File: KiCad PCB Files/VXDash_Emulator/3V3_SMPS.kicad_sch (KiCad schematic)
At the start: 13 parts, among them IC2 AP62200

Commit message: Emulator board : BOM and fab prep
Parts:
- C10: MFT (none) -> Samsung Electro-Mechanics; MFT_PN (none) -> CL31B106KAHNNNE
- C11, C12, C14: MFT (none) -> Samsung Electro-Mechanics; MFT_PN (none) -> CL10B104KB8NNWC
- C13: MFT (none) -> Kyocera AVX; MFT_PN (none) -> 06035C220JAT2A
- C15, C16: MFT (none) -> Samsung Electro-Mechanics; MFT_PN (none) -> CL31B226KPHNNNE
- R91: MFT (none) -> StackPole Electronics; MFT_PN (none) -> RMCF0603FT820K
- R92: MFT (none) -> StackPole Electronics; MFT_PN (none) -> RMCF0603FT120K
- R93: MFT (none) -> StackPole Electronics; MFT_PN (none) -> RMCF0603FT75K0
- R94: MFT (none) -> Yageo; MFT_PN (none) -> RC0603FR-1324KL
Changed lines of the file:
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@@
 			)
 		)
-		(property "Description" ""
+		(property "Description" "CAP CER 22PF 50V X7R 0603"
 			(at 168.91 66.04 0)
 			(effects
@@
 			)
 		)
-		(property "MFT" ""
+		(property "MFT" "Kyocera AVX"
 			(at 168.91 66.04 0)
 			(effects
@@
 			)
 		)
-		(property "MFT_PN" ""
+		(property "MFT_PN" "06035C220JAT2A"
 			(at 168.91 66.04 0)
 			(effects
@@
 			)
 		)
-		(property "Description" ""
+		(property "Description" "RES 24K OHM 1% 1/10W 0603"
 			(at 160.02 77.47 0)
 			(effects
@@
 			)
 		)
-		(property "MFT" ""
+		(property "MFT" "Yageo"
 			(at 160.02 77.47 0)
 			(effects
@@
 			)
 		)
-		(property "MFT_PN" ""
+		(property "MFT_PN" "RC0603FR-1324KL"
 			(at 160.02 77.47 0)
 			(effects
@@
 			)
 		)
-		(property "Description" ""
+		(property "Description" "CAP CER 10UF 25V X7R 1206"
 			(at 99.06 62.23 0)
 			(effects
@@
 			)
 		)
-		(property "MFT" ""
+		(property "MFT" "Samsung Electro-Mechanics"
 			(at 99.06 62.23 0)
 			(effects
@@
 			)
 		)
-		(property "MFT_PN" ""
+		(property "MFT_PN" "CL31B106KAHNNNE"
 			(at 99.06 62.23 0)
 			(effects
@@
 			)
 		)
-		(property "Description" ""
+		(property "Description" "RES 75K OHM 1% 1/10W 0603"
 			(at 160.02 66.04 0)
 			(effects
@@
 			)
 		)
-		(property "MFT" ""
+		(property "MFT" "StackPole Electronics"
 			(at 160.02 66.04 0)
 			(effects
@@
 			)
 		)
-		(property "MFT_PN" ""
+		(property "MFT_PN" "RMCF0603FT75K0"
 			(at 160.02 66.04 0)
 			(effects
@@
 			)
 		)
-		(property "Description" ""
+		(property "Description" "RES 820K OHM 1% 1/10W 0603"
 			(at 88.9 63.5 0)
 			(effects
@@
 			)
 		)
-		(property "MFT" ""
+		(property "MFT" "StackPole Electronics"
 			(at 88.9 63.5 0)
 			(effects
@@
 			)
 		)
-		(property "MFT_PN" ""
+		(property "MFT_PN" "RMCF0603FT820K"
 			(at 88.9 63.5 0)
 			(effects
@@
 			)
 		)
-		(property "Description" ""
+		(property "Description" "CAP CER 22UF 10V X7R 1206"
 			(at 200.66 66.04 0)
 			(effects
@@
 			)
 		)
-		(property "MFT" ""
+		(property "MFT" "Samsung Electro-Mechanics"
 			(at 200.66 66.04 0)
 			(effects
@@
 			)
 		)
-		(property "MFT_PN" ""
+		(property "MFT_PN" "CL31B226KPHNNNE"
 			(at 200.66 66.04 0)
 			(effects
@@
 			)
 		)
-		(property "Description" ""
+		(property "Description" "CAP CER 22UF 10V X7R 1206"
 			(at 193.04 66.04 0)
 			(effects
@@
 			)
 		)
-		(property "MFT" ""
+		(property "MFT" "Samsung Electro-Mechanics"
 			(at 193.04 66.04 0)
 			(effects
@@
 			)
 		)
-		(property "MFT_PN" ""
+		(property "MFT_PN" "CL31B226KPHNNNE"
 			(at 193.04 66.04 0)
 			(effects
@@
 			)
 		)
-		(property "Description" ""
+		(property "Description" "FIXED IND 3.3UH 3A 30 MOHM SMD"
 			(at 153.67 63.5 0)
 			(effects
@@
 			)
 		)
-		(property "Description" ""
+		(property "Description" "RES 120K OHM 1% 1/10W 0603"
 			(at 88.9 76.2 0)
 			(effects
@@
 			)
 		)
-		(property "MFT" ""
+		(property "MFT" "StackPole Electronics"
 			(at 88.9 76.2 0)
 			(effects
@@
 			)
 		)
-		(property "MFT_PN" ""
+		(property "MFT_PN" "RMCF0603FT120K"
 			(at 88.9 76.2 0)
 			(effects
@@
 			)
 		)
-		(property "Description" ""
+		(property "Description" "CAP CER 0.1UF 50V X7R 0603"
 			(at 106.68 62.23 0)
 			(effects
@@
 			)
 		)
-		(property "MFT" ""
+		(property "MFT" "Samsung Electro-Mechanics"
 			(at 106.68 62.23 0)
 			(effects
@@
 			)
 		)
-		(property "MFT_PN" ""
+		(property "MFT_PN" "CL10B104KB8NNWC"
 			(at 106.68 62.23 0)
 			(effects
@@
 			)
 		)
-		(property "Description" ""
+		(property "Description" "CAP CER 0.1UF 50V X7R 0603"
 			(at 140.97 55.88 0)
 			(effects
@@
 			)
 		)
-		(property "MFT" ""
+		(property "MFT" "Samsung Electro-Mechanics"
 			(at 140.97 55.88 0)
 			(effects
@@
 			)
 		)
-		(property "MFT_PN" ""
+		(property "MFT_PN" "CL10B104KB8NNWC"
 			(at 140.97 55.88 0)
 			(effects
@@
 			)
 		)
-		(property "Description" ""
+		(property "Description" "CAP CER 0.1UF 50V X7R 0603"
 			(at 185.42 66.04 0)
 			(effects
@@
 			)
 		)
-		(property "MFT" ""
+		(property "MFT" "Samsung Electro-Mechanics"
 			(at 185.42 66.04 0)
 			(effects
@@
 			)
 		)
-		(property "MFT_PN" ""
+		(property "MFT_PN" "CL10B104KB8NNWC"
 			(at 185.42 66.04 0)
 			(effects

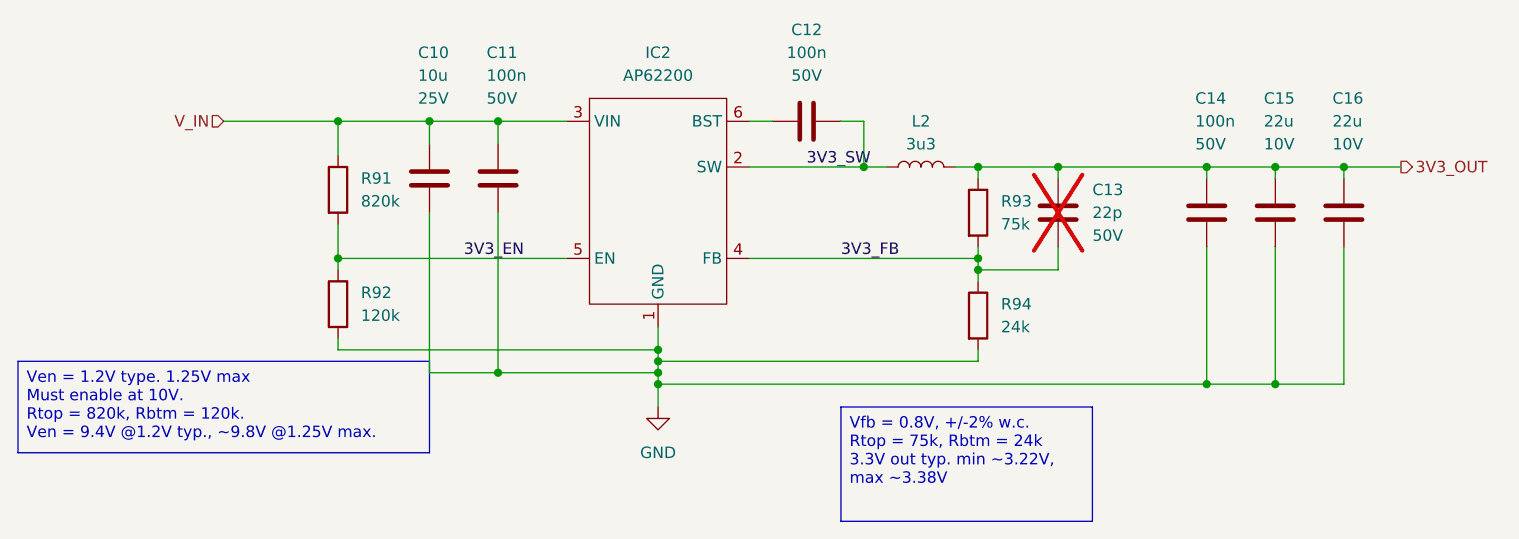
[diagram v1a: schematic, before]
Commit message: Emulator : LCSC part numbers and production files
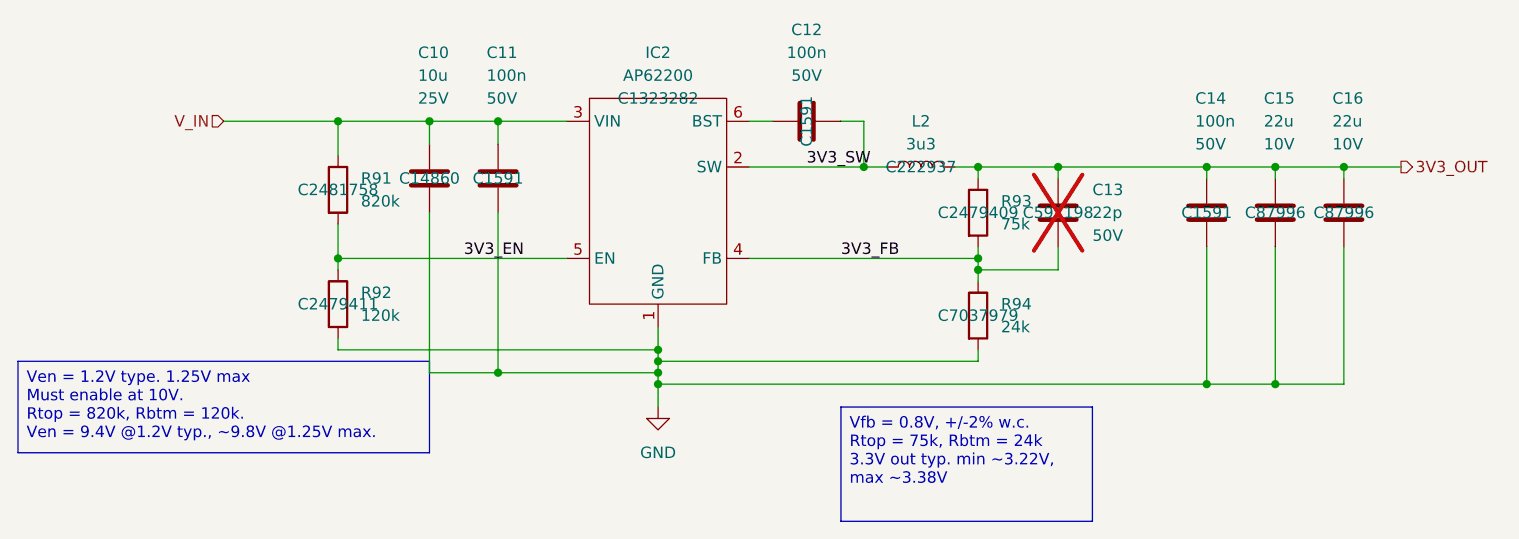
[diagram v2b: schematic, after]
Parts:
- C10: LCSC (none) -> C14860
- C11, C12, C14: LCSC (none) -> C1591; MFT_PN CL10B104KB8NNWC -> CL10B104KB8NNNC
- C13: LCSC (none) -> C597198
- C15, C16: LCSC (none) -> C87996
- IC2: LCSC (none) -> C1323282
- L2: LCSC (none) -> C222937
- R91: LCSC (none) -> C2481758
- R92: LCSC (none) -> C2479411
- R93: LCSC (none) -> C2479409
- R94: LCSC (none) -> C7037979
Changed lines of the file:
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@@
+			)
+		)
+		(property "LCSC" "C1323282"
+			(at 124.46 53.34 0)
+			(effects
+				(font
+					(size 1.27 1.27)
+				)
 			)
 		)
@@
 			)
 		)
+		(property "LCSC" "C597198"
+			(at 168.91 66.04 0)
+			(effects
+				(font
+					(size 1.27 1.27)
+				)
+			)
+		)
 		(pin "1"
 		)
@@
 			)
 		)
+		(property "LCSC" "C7037979"
+			(at 160.02 77.47 0)
+			(effects
+				(font
+					(size 1.27 1.27)
+				)
+			)
+		)
 		(pin "1"
 		)
@@
 			)
 		)
+		(property "LCSC" "C14860"
+			(at 99.06 62.23 0)
+			(effects
+				(font
+					(size 1.27 1.27)
+				)
+			)
+		)
 		(pin "1"
 		)
@@
 			)
 		)
+		(property "LCSC" "C2479409"
+			(at 160.02 66.04 0)
+			(effects
+				(font
+					(size 1.27 1.27)
+				)
+			)
+		)
 		(pin "1"
 		)
@@
 			)
 		)
+		(property "LCSC" "C2481758"
+			(at 88.9 63.5 0)
+			(effects
+				(font
+					(size 1.27 1.27)
+				)
+			)
+		)
 		(pin "1"
 		)
@@
 			)
 		)
+		(property "LCSC" "C87996"
+			(at 200.66 66.04 0)
+			(effects
+				(font
+					(size 1.27 1.27)
+				)
+			)
+		)
 		(pin "2"
 		)
@@
 				)
 				(hide yes)
+			)
+		)
+		(property "LCSC" "C87996"
+			(at 193.04 66.04 0)
+			(effects
+				(font
+					(size 1.27 1.27)
+				)
 			)
 		)
@@
 			)
 		)
+		(property "LCSC" "C222937"
+			(at 153.67 60.96 0)
+			(effects
+				(font
+					(size 1.27 1.27)
+				)
+			)
+		)
 		(pin "2"
 		)
@@
 			)
 		)
+		(property "LCSC" "C2479411"
+			(at 88.9 76.2 0)
+			(effects
+				(font
+					(size 1.27 1.27)
+				)
+			)
+		)
 		(pin "1"
 		)
@@
 			)
 		)
-		(property "MFT_PN" "CL10B104KB8NNWC"
+		(property "MFT_PN" "CL10B104KB8NNNC"
 			(at 106.68 62.23 0)
 			(effects
@@
 				)
 				(hide yes)
+			)
+		)
+		(property "LCSC" "C1591"
+			(at 106.68 62.23 0)
+			(effects
+				(font
+					(size 1.27 1.27)
+				)
 			)
 		)
@@
 			)
 		)
-		(property "MFT_PN" "CL10B104KB8NNWC"
+		(property "MFT_PN" "CL10B104KB8NNNC"
 			(at 140.97 55.88 0)
 			(effects
@@
 				)
 				(hide yes)
+			)
+		)
+		(property "LCSC" "C1591"
+			(at 140.97 55.88 0)
+			(effects
+				(font
+					(size 1.27 1.27)
+				)
 			)
 		)
@@
 			)
 		)
-		(property "MFT_PN" "CL10B104KB8NNWC"
+		(property "MFT_PN" "CL10B104KB8NNNC"
 			(at 185.42 66.04 0)
 			(effects
@@
 			)
 		)
+		(property "LCSC" "C1591"
+			(at 185.42 66.04 0)
+			(effects
+				(font
+					(size 1.27 1.27)
+				)
+			)
+		)

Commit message: Emulator : Updating BOM with LCSC alts
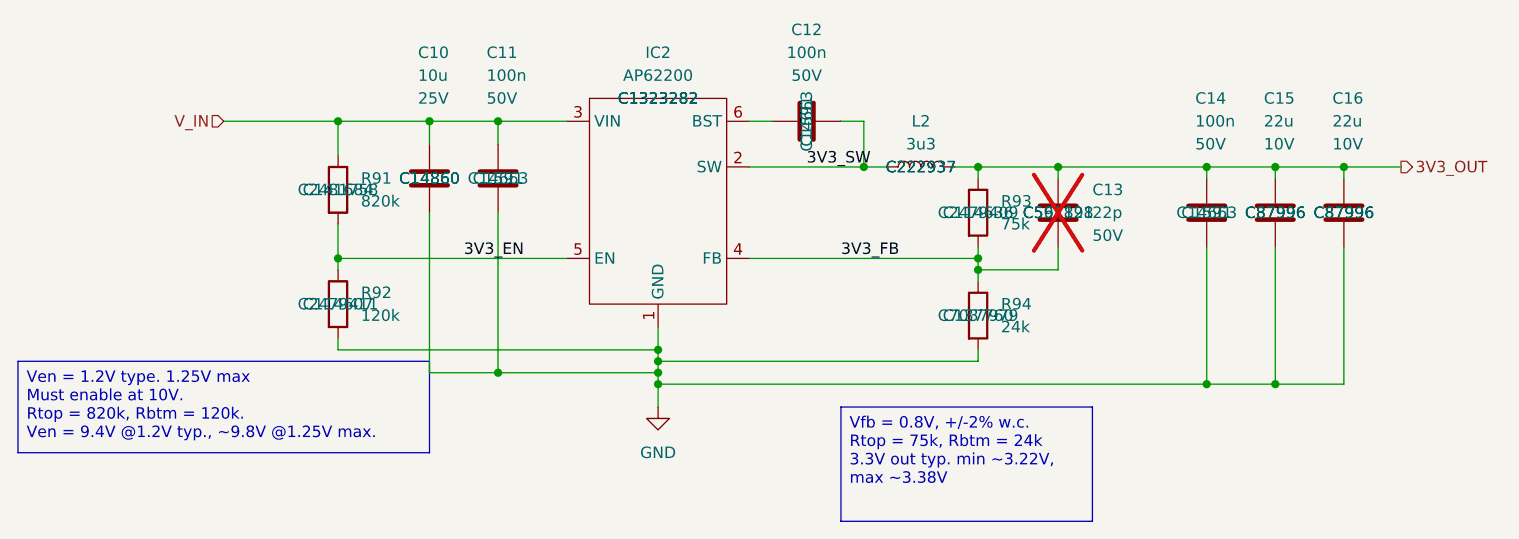
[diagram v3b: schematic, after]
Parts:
- C10: LCSC alt (none) -> C14860
- C11, C12, C14: LCSC alt (none) -> C14663
- C13: LCSC alt (none) -> C561821
- C15, C16: LCSC alt (none) -> C87996
- IC2: LCSC alt (none) -> C1323282
- L2: LCSC alt (none) -> C222937
- R91: LCSC alt (none) -> C141684
- R92: LCSC alt (none) -> C114607
- R93: LCSC alt (none) -> C114636
- R94: LCSC alt (none) -> C137760
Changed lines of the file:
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@@
+			)
+		)
+		(property "LCSC alt" "C1323282"
+			(at 124.46 53.34 0)
+			(effects
+				(font
+					(size 1.27 1.27)
+				)
 			)
 		)
@@
 			)
 		)
+		(property "LCSC alt" "C561821"
+			(at 168.91 66.04 0)
+			(effects
+				(font
+					(size 1.27 1.27)
+				)
+			)
+		)
 		(pin "1"
 		)
@@
 			)
 		)
+		(property "LCSC alt" "C137760"
+			(at 160.02 77.47 0)
+			(effects
+				(font
+					(size 1.27 1.27)
+				)
+			)
+		)
 		(pin "1"
 		)
@@
 			)
 		)
+		(property "LCSC alt" "C14860"
+			(at 99.06 62.23 0)
+			(effects
+				(font
+					(size 1.27 1.27)
+				)
+			)
+		)
 		(pin "1"
 		)
@@
 			)
 		)
+		(property "LCSC alt" "C114636"
+			(at 160.02 66.04 0)
+			(effects
+				(font
+					(size 1.27 1.27)
+				)
+			)
+		)
 		(pin "1"
 		)
@@
 			)
 		)
+		(property "LCSC alt" "C141684"
+			(at 88.9 63.5 0)
+			(effects
+				(font
+					(size 1.27 1.27)
+				)
+			)
+		)
 		(pin "1"
 		)
@@
 			)
 		)
+		(property "LCSC alt" "C87996"
+			(at 200.66 66.04 0)
+			(effects
+				(font
+					(size 1.27 1.27)
+				)
+			)
+		)
 		(pin "2"
 		)
@@
 		)
 		(property "LCSC" "C87996"
+			(at 193.04 66.04 0)
+			(effects
+				(font
+					(size 1.27 1.27)
+				)
+			)
+		)
+		(property "LCSC alt" "C87996"
 			(at 193.04 66.04 0)
 			(effects
@@
 			)
 		)
+		(property "LCSC alt" "C222937"
+			(at 153.67 60.96 0)
+			(effects
+				(font
+					(size 1.27 1.27)
+				)
+			)
+		)
 		(pin "2"
 		)
@@
 			)
 		)
+		(property "LCSC alt" "C114607"
+			(at 88.9 76.2 0)
+			(effects
+				(font
+					(size 1.27 1.27)
+				)
+			)
+		)
 		(pin "1"
 		)
@@
 		)
 		(property "LCSC" "C1591"
+			(at 106.68 62.23 0)
+			(effects
+				(font
+					(size 1.27 1.27)
+				)
+			)
+		)
+		(property "LCSC alt" "C14663"
 			(at 106.68 62.23 0)
 			(effects
@@
 			)
 		)
+		(property "LCSC alt" "C14663"
+			(at 140.97 55.88 0)
+			(effects
+				(font
+					(size 1.27 1.27)
+				)
+			)
+		)
 		(pin "1"
 		)
@@
 			(at 185.42 66.04 0)
 			(effects
+				(font
+					(size 1.27 1.27)
+				)
+			)
+		)
+		(property "LCSC alt" "C14663"
+			(at 185.42 66.04 0)
+			(effects
